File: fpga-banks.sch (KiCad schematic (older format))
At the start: 57 parts, among them J13 62000311121, Q12 2N7002, Q13 2N7002, Q14 2N7002, Q15 2N7002, Q16 2N7002, U14 XC7A100T-FGG484

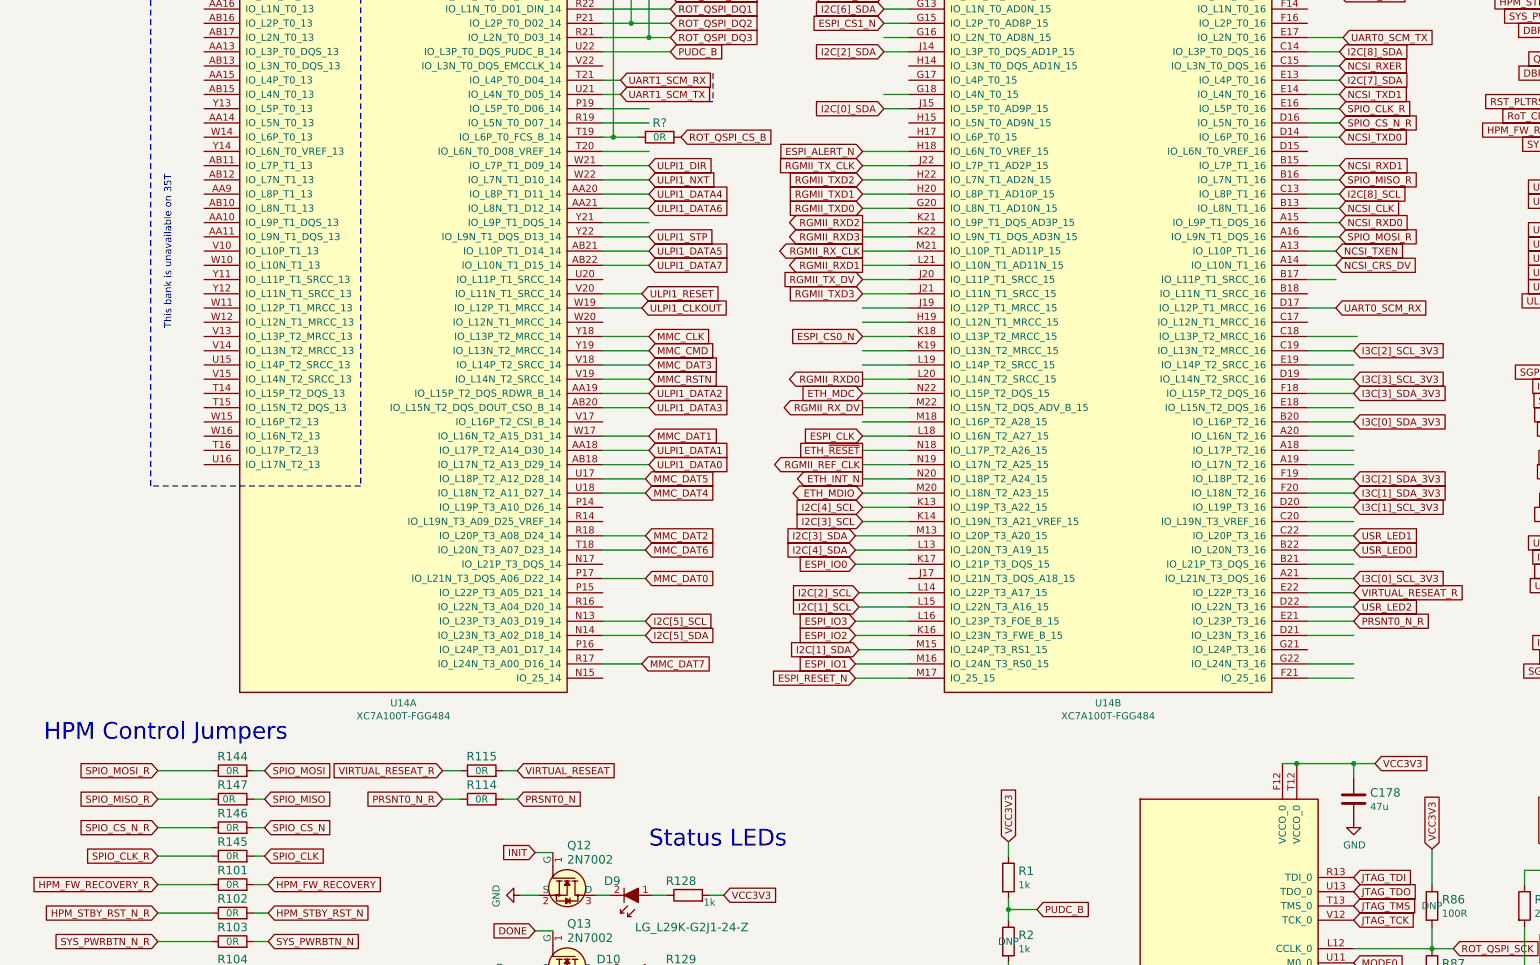
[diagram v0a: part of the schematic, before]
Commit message: Typo fix
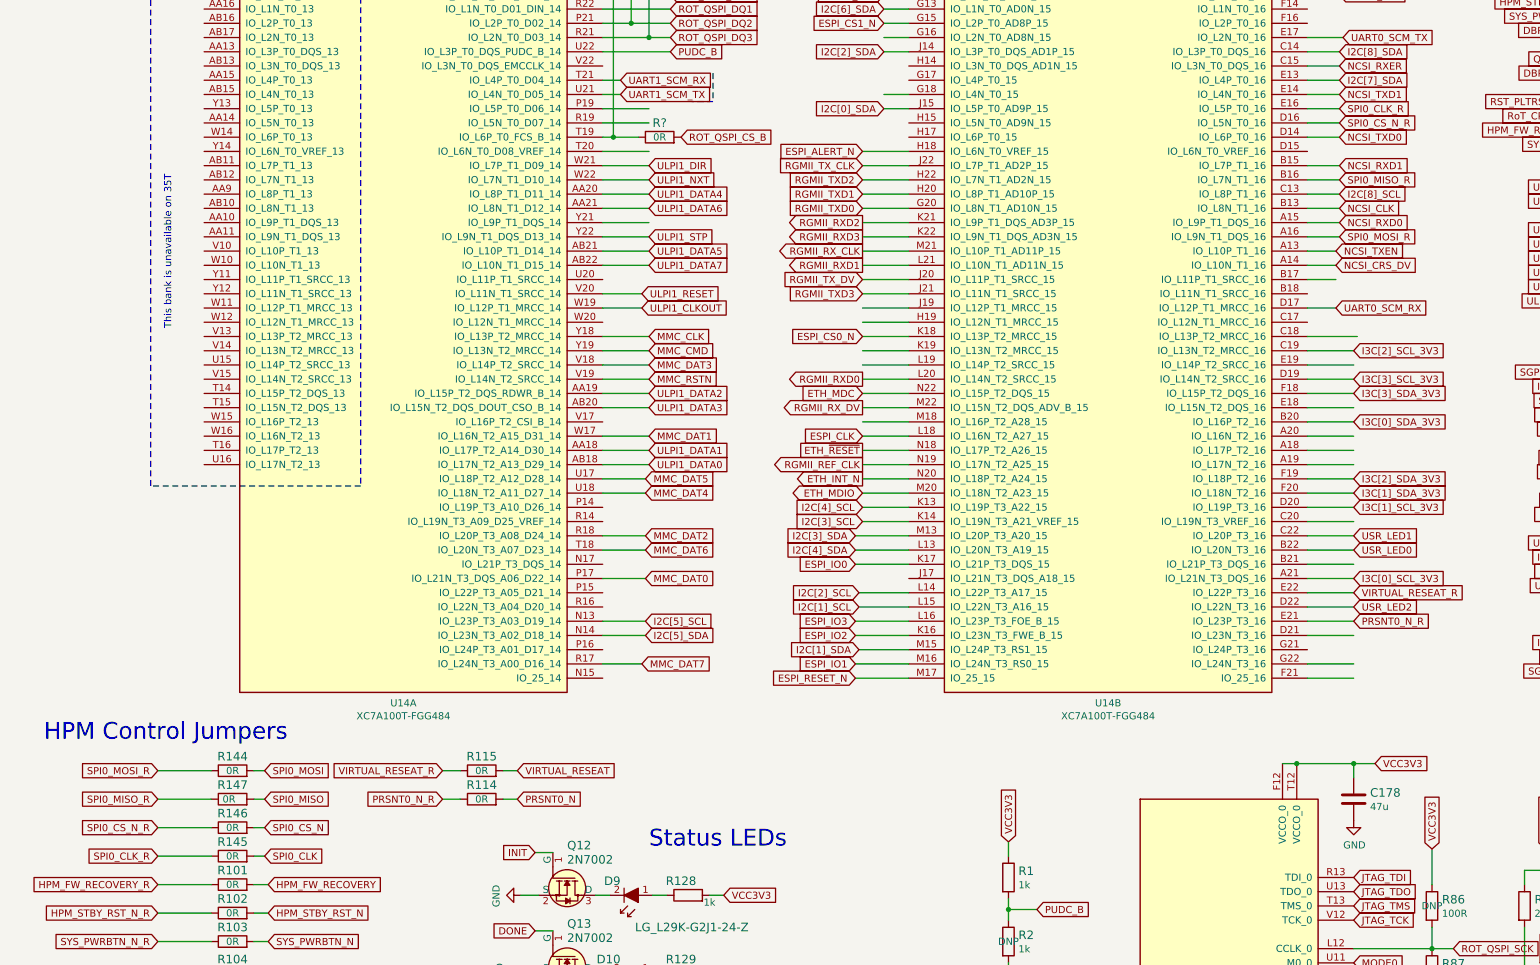
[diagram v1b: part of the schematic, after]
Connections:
- net labels added: SPI0_CLK, SPI0_CLK_R, SPI0_CS_N, SPI0_CS_N_R, SPI0_MISO, SPI0_MISO_R, SPI0_MOSI, SPI0_MOSI_R
- net labels removed: SPIO_CLK, SPIO_CLK_R, SPIO_CS_N, SPIO_CS_N_R, SPIO_MISO, SPIO_MISO_R, SPIO_MOSI, SPIO_MOSI_R
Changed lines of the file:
@@
 	3850 7600 3950 7600
 Text GLabel 2175 8200 2    50   Input ~ 0
-SPIO_CLK
+SPI0_CLK
 Text GLabel 2175 8000 2    50   Input ~ 0
-SPIO_CS_N
+SPI0_CS_N
 Text GLabel 2175 7600 2    50   Input ~ 0
-SPIO_MOSI
+SPI0_MOSI
 Text GLabel 2175 7800 2    50   Input ~ 0
-SPIO_MISO
+SPI0_MISO
 Wire Wire Line
 	11600 3200 12000 3200
@@
 	6325 6950 6700 6950
 Text GLabel 1425 8200 0    50   Input ~ 0
-SPIO_CLK_R
+SPI0_CLK_R
 Text GLabel 1425 8000 0    50   Input ~ 0
-SPIO_CS_N_R
+SPI0_CS_N_R
 Text GLabel 1425 7600 0    50   Input ~ 0
-SPIO_MOSI_R
+SPI0_MOSI_R
 Text GLabel 1425 7800 0    50   Input ~ 0
-SPIO_MISO_R
+SPI0_MISO_R
 Wire Wire Line
 	1425 7600 1800 7600
@@
 	1425 8200 1800 8200
 Text GLabel 9725 2950 2    50   Input ~ 0
-SPIO_CLK_R
+SPI0_CLK_R
 Text GLabel 9725 3050 2    50   Input ~ 0
-SPIO_CS_N_R
+SPI0_CS_N_R
 Text GLabel 9725 3850 2    50   Input ~ 0
-SPIO_MOSI_R
+SPI0_MOSI_R
 Text GLabel 9725 3450 2    50   Input ~ 0
-SPIO_MISO_R
+SPI0_MISO_R
 Wire Wire Line
 	9500 3450 9725 3450
